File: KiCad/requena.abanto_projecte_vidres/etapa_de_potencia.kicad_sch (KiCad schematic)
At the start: 11 parts, among them U1 VNH5019A-E

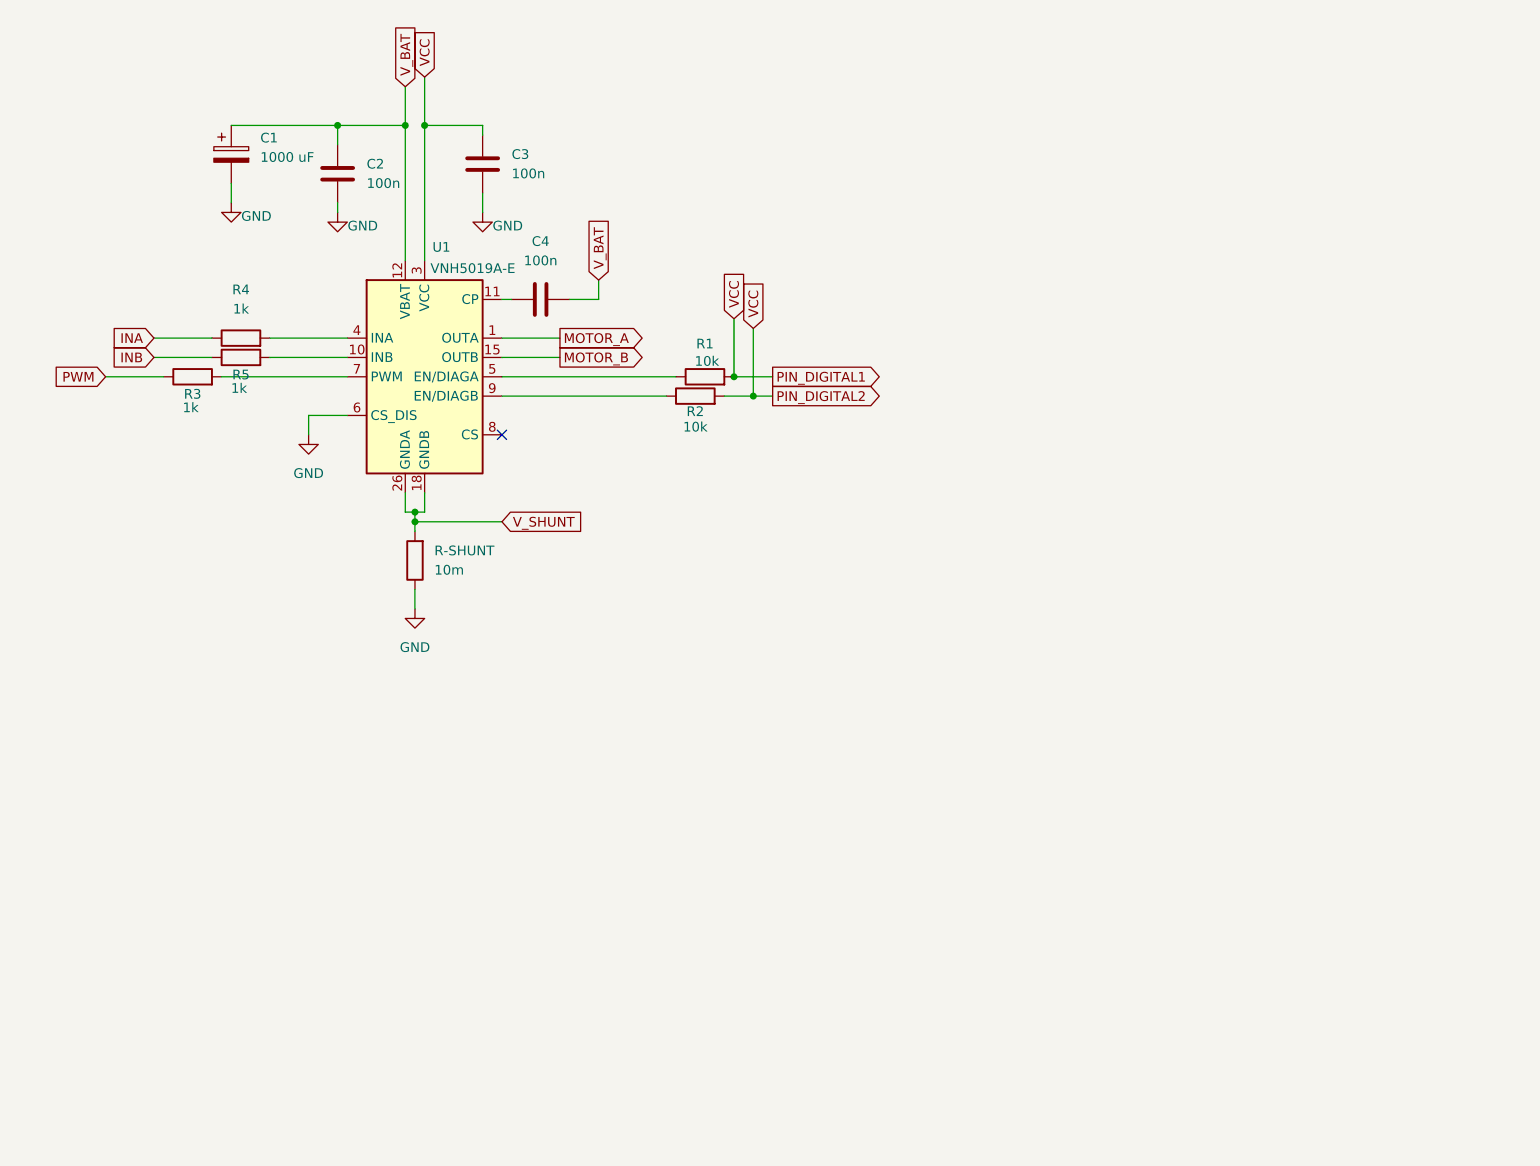
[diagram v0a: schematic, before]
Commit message: Millora projecte 1
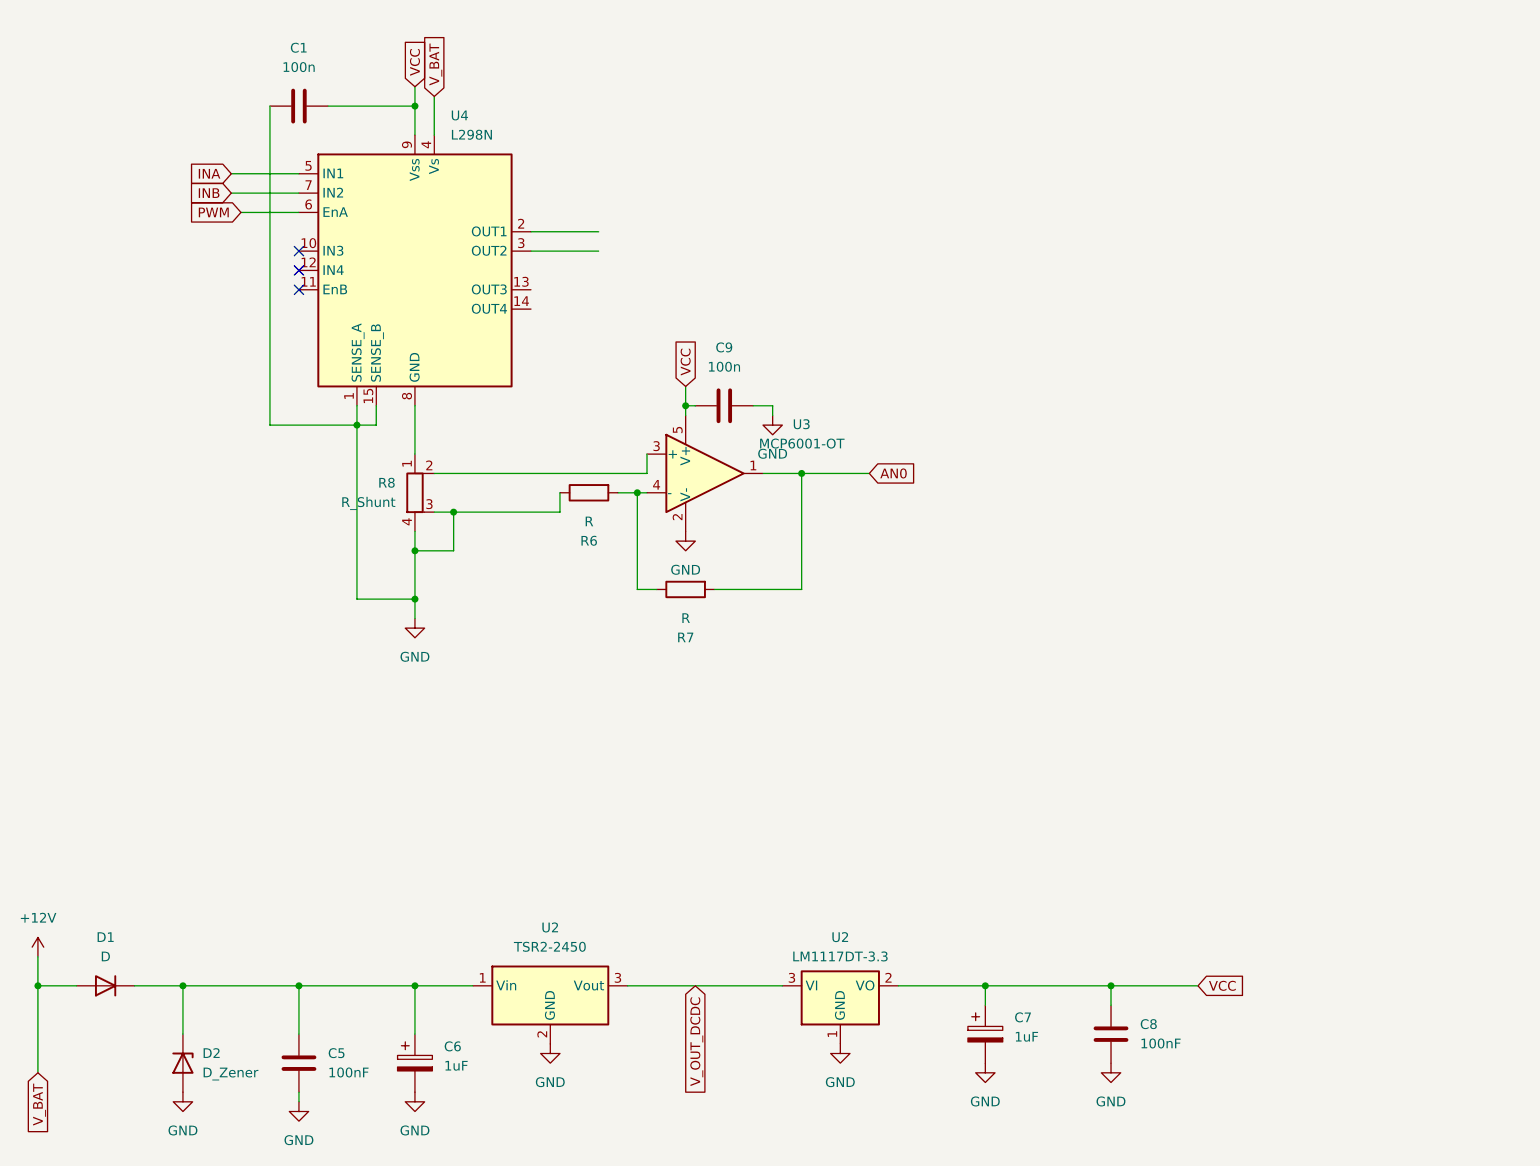
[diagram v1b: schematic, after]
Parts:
- removed C1: 1000 uF, symbol Device:C_Polarized
- removed C2, C3, C4: 100n, symbol Device:C
- removed R-SHUNT: 10m, symbol Device:R
- removed R1, R2: 10k, symbol Device:R
- removed R3, R4, R5: 1k, symbol Device:R
- removed U1: VNH5019A-E, Package_SO:ST_MultiPowerSO-30, symbol Driver_Motor:VNH5019A-E
- added C1, C9: 100n, symbol Device:C
- added C5, C8: 100nF, symbol Device:C
- added C6, C7: 1uF, symbol Device:C_Polarized
- added D1: D, symbol Device:D
- added D2: D_Zener, symbol Device:D_Zener
- added R6, R7: R, symbol Device:R
- added R8: R_Shunt, symbol Device:R_Shunt
- added U2: LM1117DT-3.3, Package_TO_SOT_SMD:TO-252-3_TabPin2, symbol Regulator_Linear:LM1117DT-3.3
- added U2: TSR2-2450, Converter_DCDC:Converter_DCDC_TRACO_TSR2-xxxx_THT, symbol Converter_DCDC:TSR2-2450
- added U3: MCP6001-OT, Package_TO_SOT_SMD:SOT-23-5, symbol Amplifier_Operational:MCP6001-OT
- added U4: L298N, Package_TO_SOT_THT:TO-220-15_P2.54x5.08mm_StaggerOdd_Lead4.58mm_Vertical, symbol Driver_Motor:L298N
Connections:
- net GND: now also C1.1, C5.2, C6.2, C7.2, C8.2, C9.2, D2.2 (A), R6.1, R8.3, R8.4, U2.1 (GND), U2.2 (GND), U3.2 (V-), U4.1 (SENSE_A), U4.15 (SENSE_B)
- net INA: now also U4.5 (IN1)
- net INB: now also U4.7 (IN2)
- net PWM: now also U4.6 (EnA)
- new net: C5.1, C6.1, D1.1 (K), D2.1 (K), U2.1 (Vin)
- new net: R6.2, R7.1, U3.4 (-)
- new net: R8.1, U4.8 (GND)
- new net: R8.2, U3.3 (+)
- new net +12V: D1.2 (A), U4.4 (Vs)
- new net AN0: R7.2, U3.1
- new net VCC: C1.2, C7.1, C8.1, C9.1, U2.2 (VO), U3.5 (V+), U4.9 (Vss)
- new net V_OUT_DCDC: U2.3 (VI), U2.3 (Vout)
- no-connect marks 1 -> 3

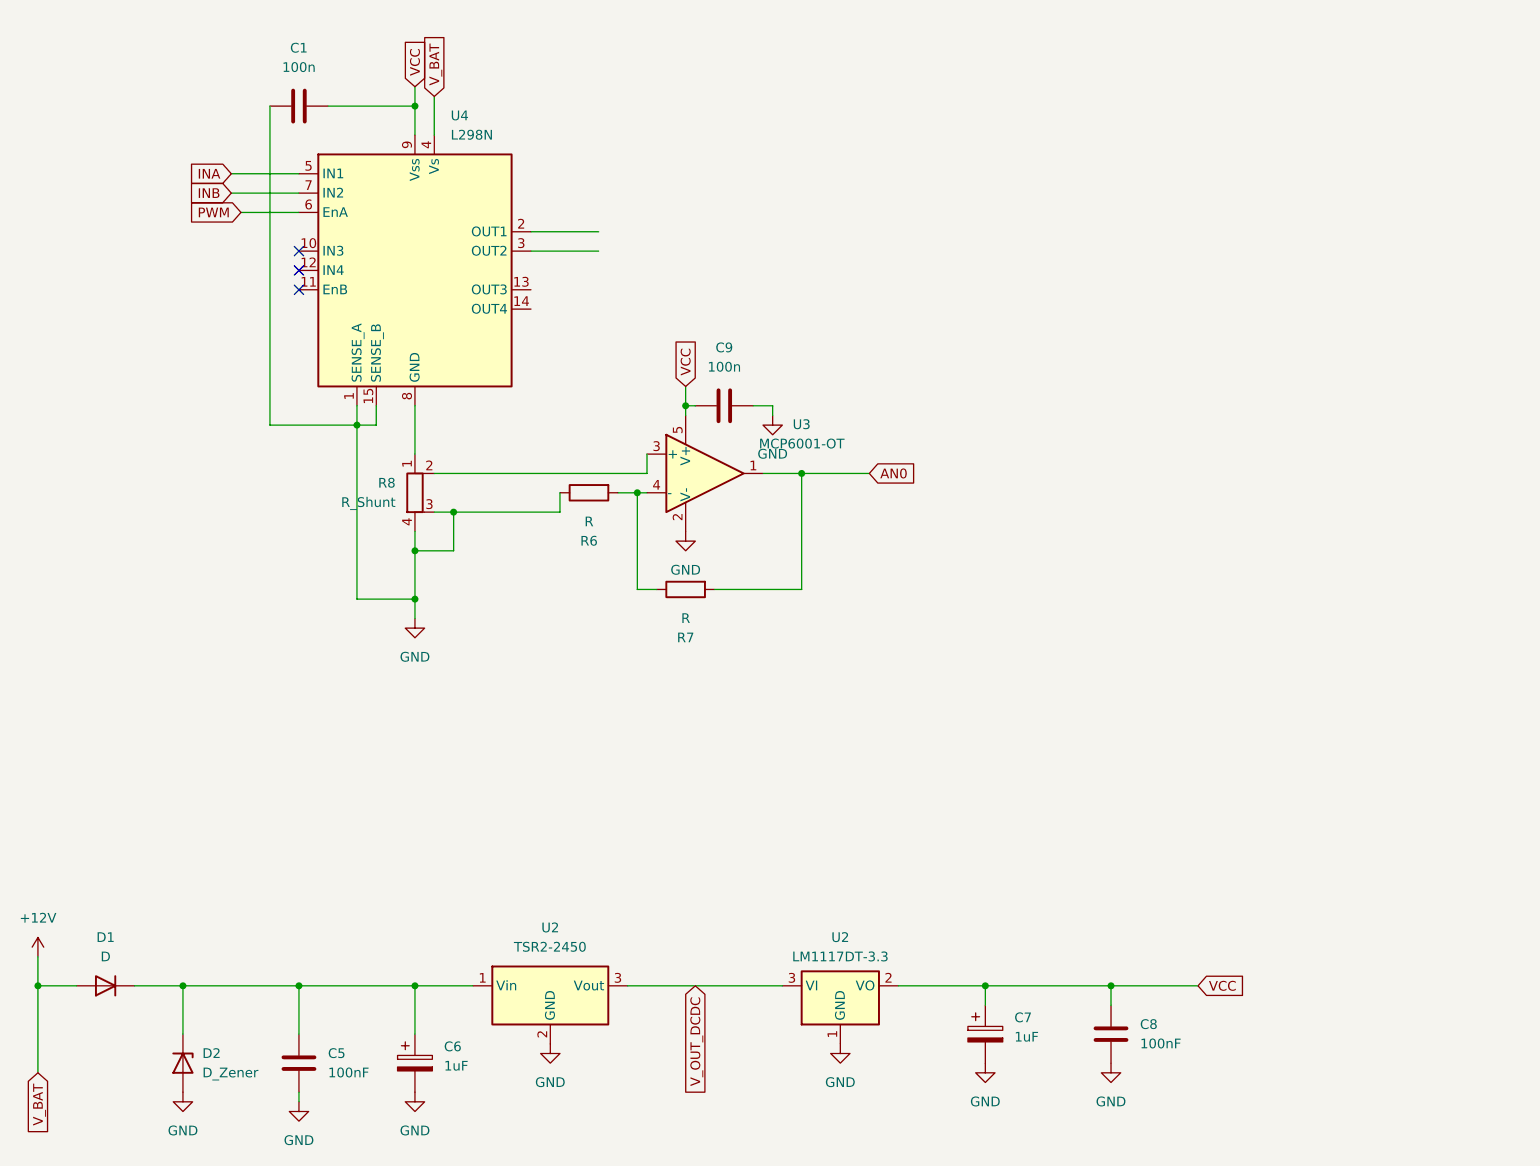
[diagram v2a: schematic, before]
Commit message: cambios
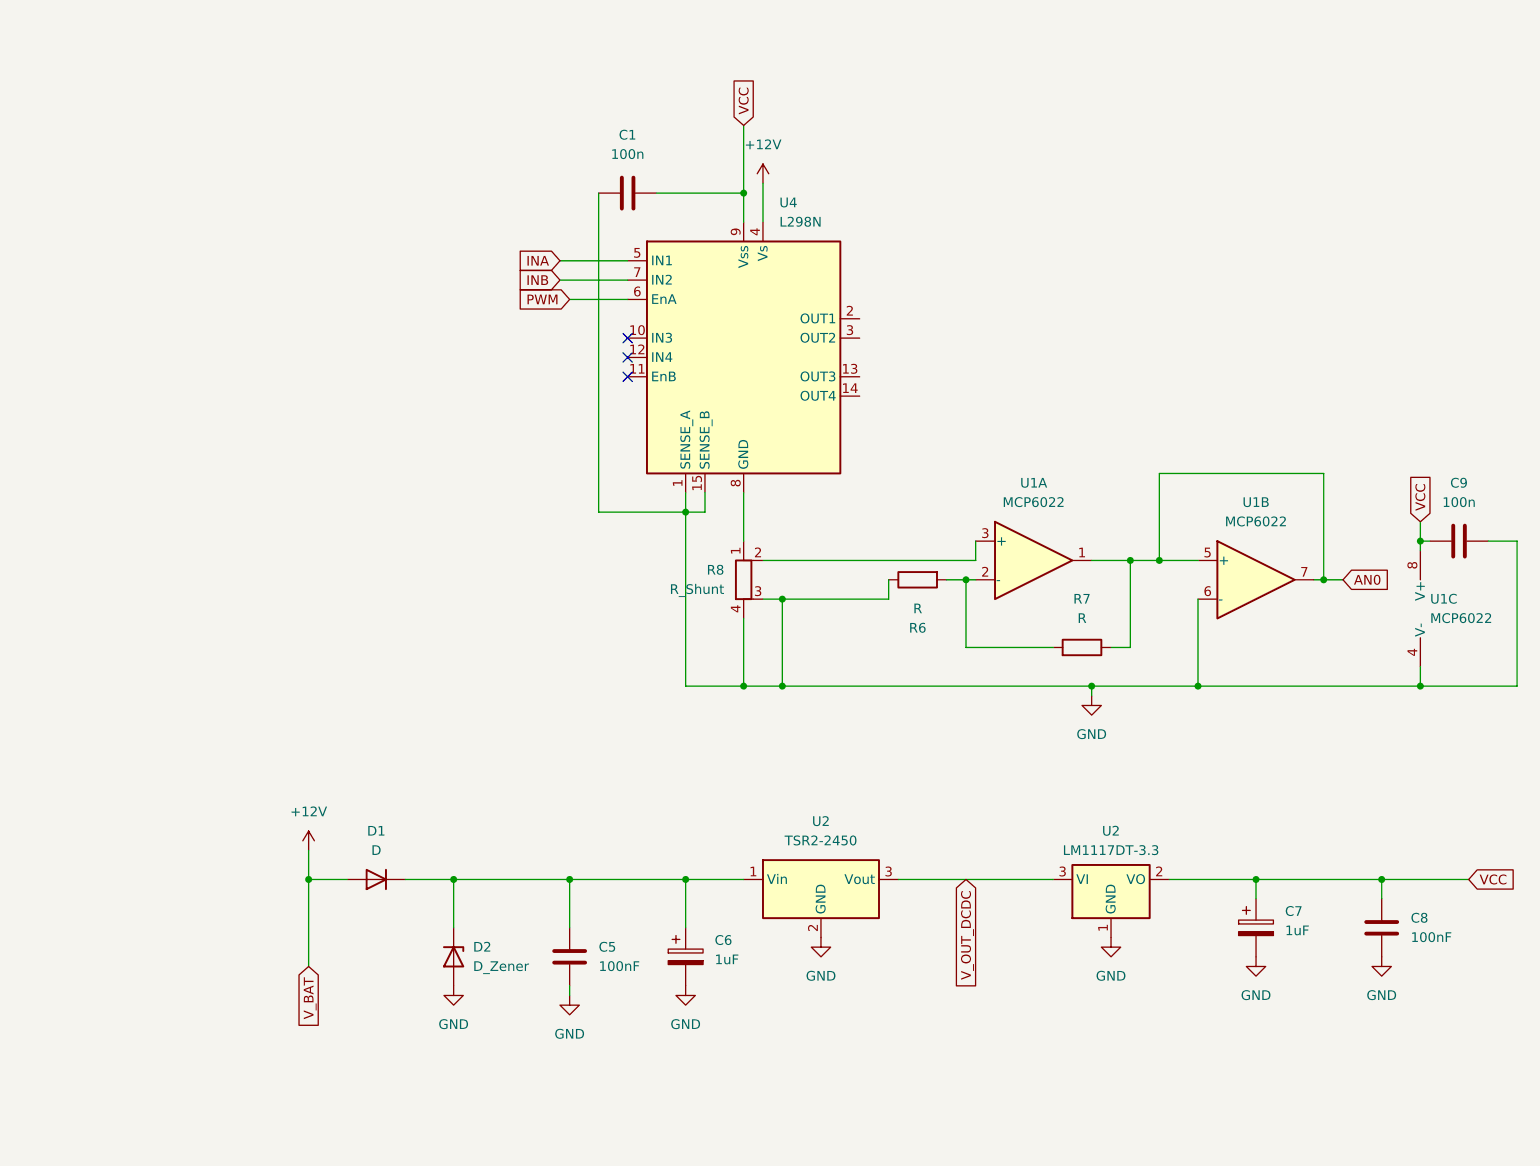
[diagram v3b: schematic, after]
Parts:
- removed U3: MCP6001-OT, Package_TO_SOT_SMD:SOT-23-5, symbol Amplifier_Operational:MCP6001-OT
- added U1: MCP6022, symbol Amplifier_Operational:MCP6022
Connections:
- net AN0: now also R7.1, U1.1, U1.5 (+), U1.7; no longer R7.2
- net GND: now also U1.4 (V-), U1.6 (-)
- net VCC: now also U1.8 (V+)
- net at R6.2: now also R7.2, U1.2 (-); no longer R7.1
- net at R8.2: now also U1.3 (+)
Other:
- moved on the sheet: C1, C5, C6, C7, C8, C9, D1, D2, R6, R7, R8, U2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
